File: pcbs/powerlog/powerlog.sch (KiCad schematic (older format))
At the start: 40 parts, among them J1 Conn_01x06, J2 USB_B_Micro, J3 Conn_01x06, J4 TC2030, SW1 SW_Push, U1 AP2112K-3.3, U2 INA3221, U4 ATSAMD21E15B-M

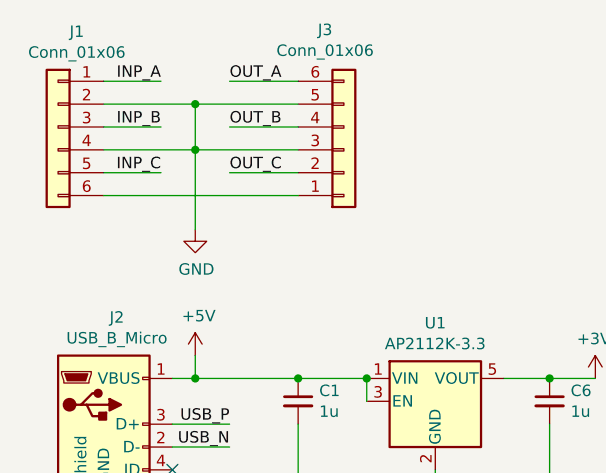
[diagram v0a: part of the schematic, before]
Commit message: Layout
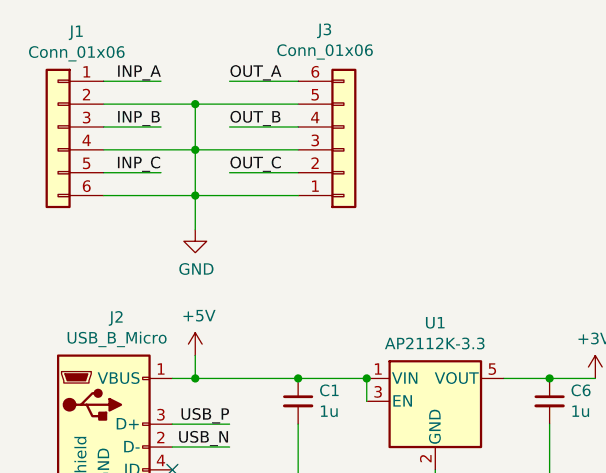
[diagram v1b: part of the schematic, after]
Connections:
- net GND: now also J1.6 (Pin_6), J3.1 (Pin_1)
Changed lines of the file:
@@
 $EndComp
 Wire Wire Line
-	1050 1350 1900 1350
+	1050 1350 1450 1350
 Wire Wire Line
-	1450 1150 1450 1500
+	1450 1150 1450 1350
 Wire Wire Line
 	1050 1250 1300 1250
@@
 	-1   0    0    -1
 $EndComp
+Connection ~ 1450 1350
+Wire Wire Line
+	1450 1350 1900 1350
+Wire Wire Line
+	1450 1350 1450 1500
 $EndSCHEMATC

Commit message: Update powerlog
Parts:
- U4: symbol MCU_Microchip_SAMD:ATSAMD21E15B-M -> powerlog-rescue:ATSAMD21E15B-M-MCU_Microchip_SAMD
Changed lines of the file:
@@
 Connection ~ 3000 2150
 $Comp
-L MCU_Microchip_SAMD:ATSAMD21E15B-M U4
+L powerlog-rescue:ATSAMD21E15B-M-MCU_Microchip_SAMD U4
 U 1 1 60175019
 P 8650 3250
